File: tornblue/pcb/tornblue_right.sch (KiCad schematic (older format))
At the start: 80 parts, among them J1 BATT, J2 SWD, J3 BREAKOUT, J4 USB C - USB2.0, J5 BATT_PIN, Q1 AO3401A, Q2 AO3401A, SW1 SW_Push, SW10 SW_Push, SW11 SW_Push, SW12 SW_Push, SW13 SW_Push, SW14 SW_Push, SW15 SW_Push, SW16 SW_Push, SW17 SW_Push, SW18 SW_Push, SW19 EC11, SW2 SW_Push, SW20 SW_Push, SW21 SW_Push, SW22 EC11, SW23 RESET, SW24 SW_SPST, SW3 SW_Push, SW4 SW_Push, SW5 SW_Push, SW6 SW_Push, SW7 SW_Push, SW8 SW_Push, SW9 SW_Push, U1 XC6220, U2 TP4056, U3 nRF52840_holyiot_18010, U4 SRV05-4

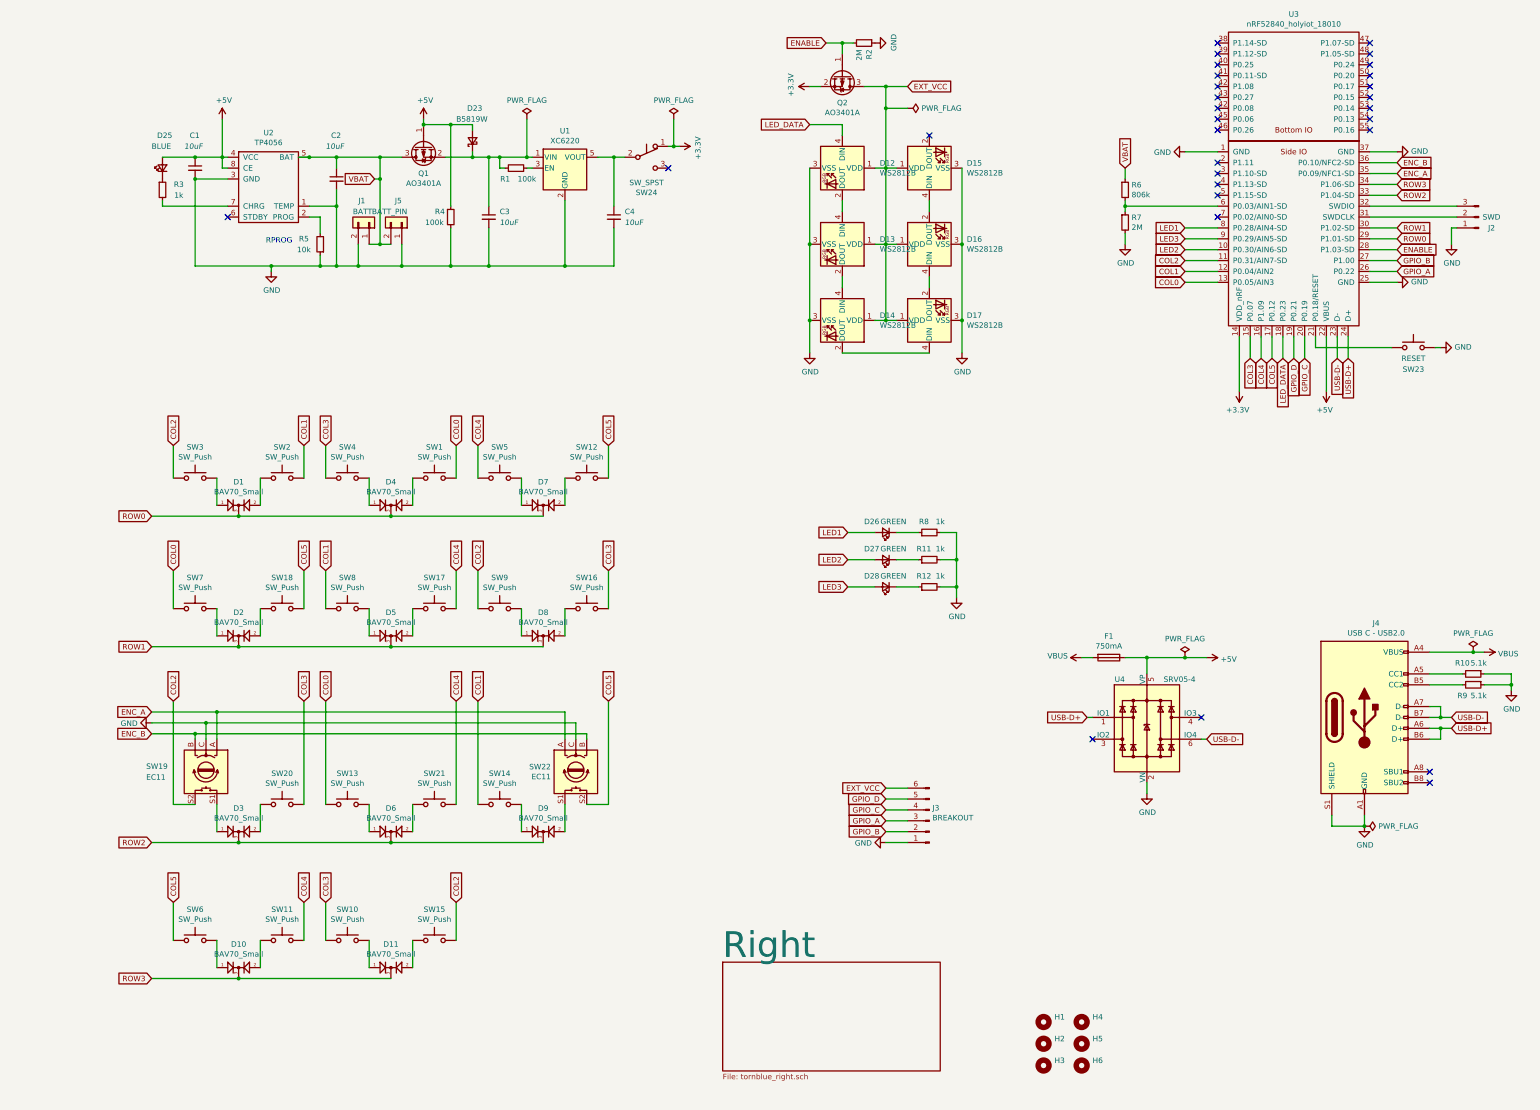
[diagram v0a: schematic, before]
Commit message: Add right schematic
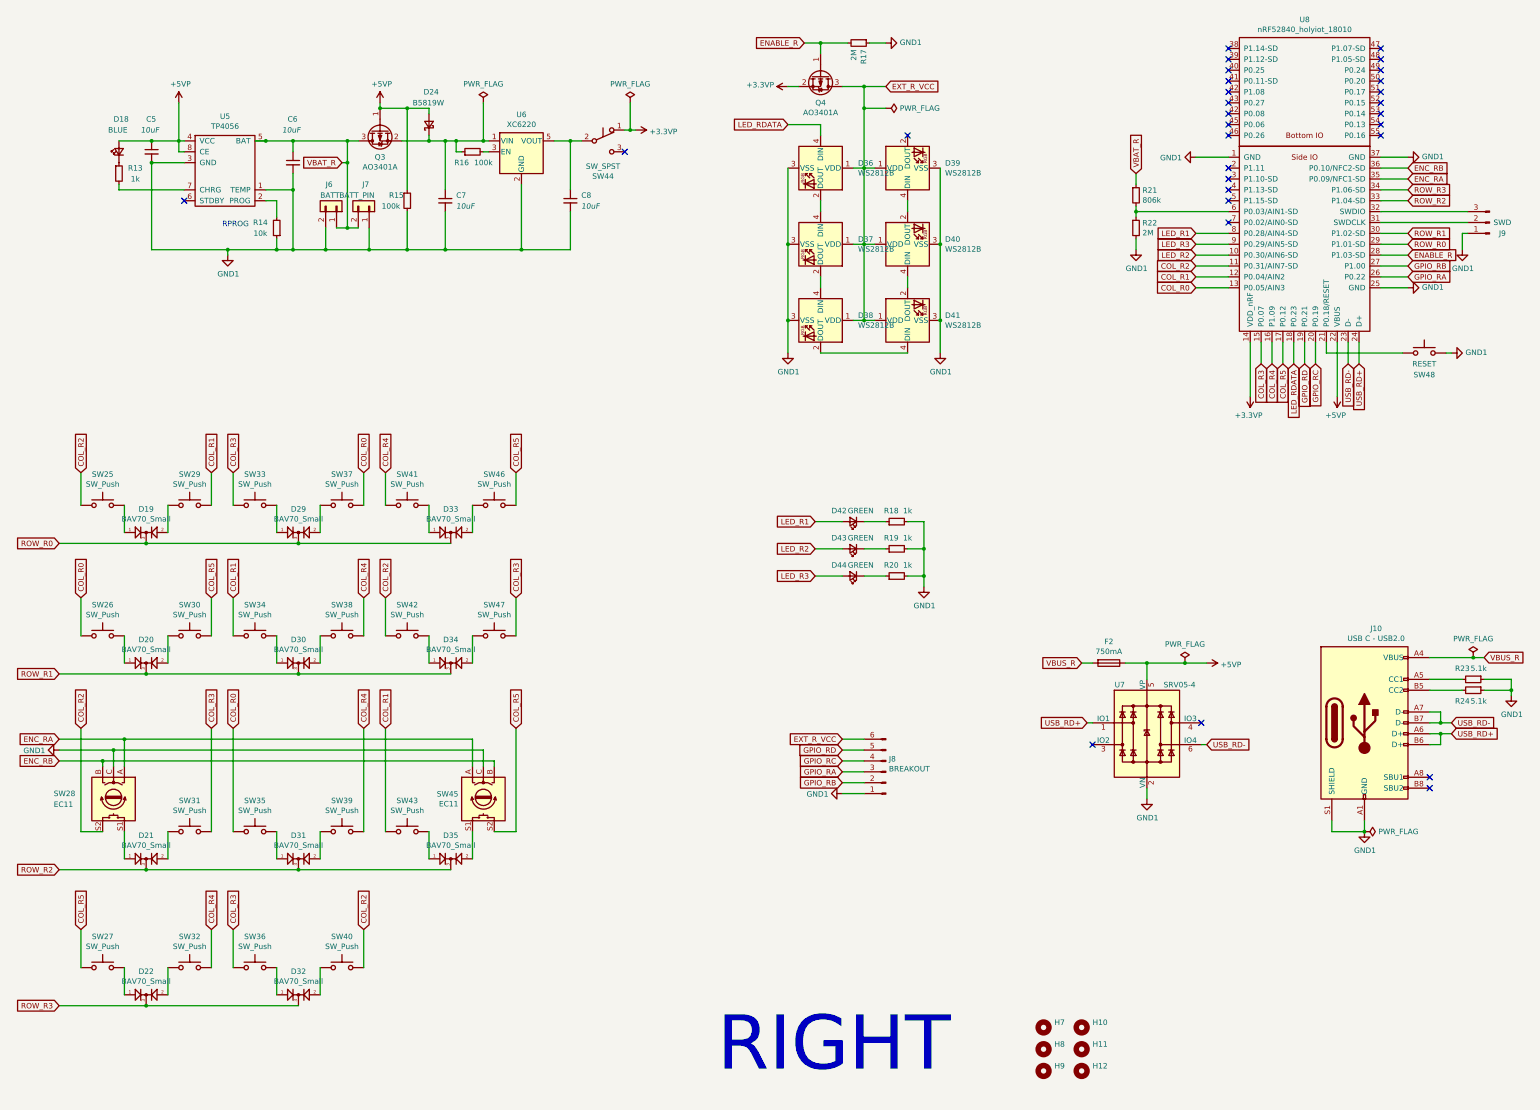
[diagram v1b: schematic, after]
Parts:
- removed C1, C2, C3, C4: 10uF, Diode_SMD:D_0805_2012Metric, symbol Device:C_Small
- removed D1, D10, D11, D2, D3, D4, D5, D6, D7, D8, D9: BAV70_Small, Package_TO_SOT_SMD:SOT-23, symbol kicad-keyboard-parts:BAV70_Small
- removed D12, D13, D14, D15, D16, D17: WS2812B, LED_SMD:LED_WS2812B_PLCC4_5.0x5.0mm_P3.2mm, symbol LED:WS2812B
- removed D23: B5819W, Diode_SMD:D_SOD-123, symbol Device:D_Schottky_Small
- removed D25: BLUE, LED_SMD:LED_0805_2012Metric, symbol Device:LED_Small
- removed D26, D27, D28: GREEN, LED_SMD:LED_0805_2012Metric, symbol Device:LED_Small
- removed F1: 750mA, Fuse:Fuse_1206_3216Metric, symbol Device:Fuse
- removed H1, H2, H3, H4: MountingHole, MountingHole:MountingHole_3.2mm_M3_DIN965_Pad, symbol Mechanical:MountingHole
- removed H5, H6: MountingHole, tornblue:MountingHole_3.2mm_M3_DIN965_Pad_Slot, symbol Mechanical:MountingHole
- removed J1: BATT, Connector_JST:JST_PH_S2B-PH-SM4-TB_1x02-1MP_P2.00mm_Horizontal, symbol Connector_Generic:Conn_01x02
- removed J2: SWD, tornblue:SOIC_clipProgSmall, symbol Connector:Conn_01x03_Male
- removed J3: BREAKOUT, Connector_PinHeader_1.27mm:PinHeader_1x06_P1.27mm_Vertical, symbol Connector:Conn_01x06_Male
- removed J4: USB C - USB2.0, Connector_USB:USB_C_Receptacle_XKB_U262-16XN-4BVC11, symbol Connector:USB_C_Receptacle_USB2.0
- removed J5: BATT_PIN, Connector_PinHeader_2.54mm:PinHeader_1x02_P2.54mm_Vertical, symbol Connector_Generic:Conn_01x02
- removed Q1, Q2: AO3401A, Package_TO_SOT_SMD:SOT-23, symbol Transistor_FET:AO3401A
- removed R1, R4: 100k, Resistor_SMD:R_0805_2012Metric, symbol Device:R_Small
- removed R10, R9: 5.1k, Resistor_SMD:R_0805_2012Metric, symbol Device:R_Small
- removed R11, R12, R3, R8: 1k, Resistor_SMD:R_0805_2012Metric, symbol Device:R_Small
- removed R2, R7: 2M, Resistor_SMD:R_0805_2012Metric, symbol Device:R_Small
- removed R5: 10k, Resistor_SMD:R_0805_2012Metric, symbol Device:R_Small
- removed R6: 806k, Resistor_SMD:R_0805_2012Metric, symbol Device:R_Small
- removed SW1, SW10, SW11, SW12, SW13, SW14, SW15, SW16, SW17, SW18, SW2, SW20, SW21, SW3, SW4, SW5, SW6, SW7, SW8, SW9: SW_Push, tornblue:MX_PG1350_optional, symbol Switch:SW_Push
- removed SW19, SW22: EC11, tornblue:MX_PG1350_EVQWGD001_LR_optional, symbol Device:Rotary_Encoder_Switch
- removed SW23: RESET, tornblue:SW_SPST_TS24CA, symbol Switch:SW_Push
- removed SW24: SW_SPST, Button_Switch_SMD:SW_SPDT_PCM12, symbol Switch:SW_Push_SPDT
- removed U1: XC6220, Package_TO_SOT_SMD:SOT-23-5, symbol Regulator_Linear:AP2112K-3.3
- removed U2: TP4056, Package_SO:SOIC-8-1EP_3.9x4.9mm_P1.27mm_EP2.29x3mm_ThermalVias, symbol kicad-keyboard-parts:TP4056
- removed U3: nRF52840_holyiot_18010, kicad-keyboard-parts:nRF52840_holyiot_18010, symbol tornblue-rescue:nRF52840_holyiot_18010-tornblue-tornblue-rescue
- removed U4: SRV05-4, Package_TO_SOT_SMD:SOT-23-6, symbol Power_Protection:SRV05-4
- added C5, C6, C7, C8: 10uF, Diode_SMD:D_0805_2012Metric, symbol Device:C_Small
- added D18: BLUE, LED_SMD:LED_0805_2012Metric, symbol Device:LED_Small
- added D19, D20, D21, D22, D29, D30, D31, D32, D33, D34, D35: BAV70_Small, Package_TO_SOT_SMD:SOT-23, symbol kicad-keyboard-parts:BAV70_Small
- added D24: B5819W, Diode_SMD:D_SOD-123, symbol Device:D_Schottky_Small
- added D36, D37, D38, D39, D40, D41: WS2812B, LED_SMD:LED_WS2812B_PLCC4_5.0x5.0mm_P3.2mm, symbol LED:WS2812B
- added D42, D43, D44: GREEN, LED_SMD:LED_0805_2012Metric, symbol Device:LED_Small
- added F2: 750mA, Fuse:Fuse_1206_3216Metric, symbol Device:Fuse
- added H10, H7, H8, H9: MountingHole, MountingHole:MountingHole_3.2mm_M3_DIN965_Pad, symbol Mechanical:MountingHole
- added H11, H12: MountingHole, tornblue:MountingHole_3.2mm_M3_DIN965_Pad_Slot, symbol Mechanical:MountingHole
- added J10: USB C - USB2.0, Connector_USB:USB_C_Receptacle_XKB_U262-16XN-4BVC11, symbol Connector:USB_C_Receptacle_USB2.0
- added J6: BATT, Connector_JST:JST_PH_S2B-PH-SM4-TB_1x02-1MP_P2.00mm_Horizontal, symbol Connector_Generic:Conn_01x02
- added J7: BATT_PIN, Connector_PinHeader_2.54mm:PinHeader_1x02_P2.54mm_Vertical, symbol Connector_Generic:Conn_01x02
- added J8: BREAKOUT, Connector_PinHeader_1.27mm:PinHeader_1x06_P1.27mm_Vertical, symbol Connector:Conn_01x06_Male
- added J9: SWD, tornblue:SOIC_clipProgSmall, symbol Connector:Conn_01x03_Male
- added Q3, Q4: AO3401A, Package_TO_SOT_SMD:SOT-23, symbol Transistor_FET:AO3401A
- added R13, R18, R19, R20: 1k, Resistor_SMD:R_0805_2012Metric, symbol Device:R_Small
- added R14: 10k, Resistor_SMD:R_0805_2012Metric, symbol Device:R_Small
- added R15, R16: 100k, Resistor_SMD:R_0805_2012Metric, symbol Device:R_Small
- added R17, R22: 2M, Resistor_SMD:R_0805_2012Metric, symbol Device:R_Small
- added R21: 806k, Resistor_SMD:R_0805_2012Metric, symbol Device:R_Small
- added R23, R24: 5.1k, Resistor_SMD:R_0805_2012Metric, symbol Device:R_Small
- added SW25, SW26, SW27, SW29, SW30, SW31, SW32, SW33, SW34, SW35, SW36, SW37, SW38, SW39, SW40, SW41, SW42, SW43, SW46, SW47: SW_Push, tornblue:MX_PG1350_optional, symbol Switch:SW_Push
- added SW28, SW45: EC11, tornblue:MX_PG1350_EVQWGD001_LR_optional, symbol Device:Rotary_Encoder_Switch
- added SW44: SW_SPST, Button_Switch_SMD:SW_SPDT_PCM12, symbol Switch:SW_Push_SPDT
- added SW48: RESET, tornblue:SW_SPST_TS24CA, symbol Switch:SW_Push
- added U5: TP4056, Package_SO:SOIC-8-1EP_3.9x4.9mm_P1.27mm_EP2.29x3mm_ThermalVias, symbol kicad-keyboard-parts:TP4056
- added U6: XC6220, Package_TO_SOT_SMD:SOT-23-5, symbol Regulator_Linear:AP2112K-3.3
- added U7: SRV05-4, Package_TO_SOT_SMD:SOT-23-6, symbol Power_Protection:SRV05-4
- added U8: nRF52840_holyiot_18010, kicad-keyboard-parts:nRF52840_holyiot_18010, symbol tornblue-rescue:nRF52840_holyiot_18010-tornblue-tornblue-rescue
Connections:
- new net: SW48.1, U8.21 (P0.18/RESET)
- new net: J9.2 (Pin_2), U8.31 (SWDCLK)
- new net: J9.3 (Pin_3), U8.32 (SWDIO)
- new net: R21.2, R22.1, U8.6 (P0.03/AIN1-SD)
- new net: D42.1 (K), R18.1
- new net: D43.1 (K), R19.1
- new net: D44.1 (K), R20.1
- new net: J10.B5 (CC2), R24.2
- new net: J10.A5 (CC1), R23.2
- new net: D18.1 (K), R13.1
- new net: R13.2, U5.7 (CHRG)
- new net: R14.2, U5.2 (PROG)
- new net: C7.1, D24.1 (K), Q3.2 (S), R16.1, U6.1 (VIN)
- new net: R16.2, U6.3 (EN)
- new net: C8.1, SW44.2 (B), U6.5 (VOUT)
- new net: D36.2 (DOUT), D37.4 (DIN)
- new net: D37.2 (DOUT), D38.4 (DIN)
- new net: D38.2 (DOUT), D41.4 (DIN)
- new net: D40.4 (DIN), D41.2 (DOUT)
- new net: D39.4 (DIN), D40.2 (DOUT)
- new net: D22.1 (A1), SW27.2
- new net: D22.2 (A2), SW32.2
- new net: D30.2 (A2), SW38.2
- new net: D20.2 (A2), SW30.2
- new net: D35.2 (A2), SW45.S1
- new net: D30.1 (A1), SW34.2
- new net: D31.1 (A1), SW35.2
- new net: D31.2 (A2), SW39.2
- new net: D35.1 (A1), SW43.2
- new net: D21.1 (A1), SW28.S1
- new net: D34.1 (A1), SW42.2
- new net: D20.1 (A1), SW26.2
- new net: D21.2 (A2), SW31.2
- new net: D19.1 (A1), SW25.2
- new net: D19.2 (A2), SW29.2
- new net: D33.1 (A1), SW41.2
- new net: D33.2 (A2), SW46.2
- new net: D29.1 (A1), SW33.2
- new net: D29.2 (A2), SW37.2
- new net: D32.2 (A2), SW40.2
- new net: D34.2 (A2), SW47.2
- new net: D32.1 (A1), SW36.2
- new net +3.3VP: Q4.2 (S), SW44.1 (A), U8.14 (VDD_nRF)
- new net +5VP: C5.1, D18.2 (A), D24.2 (A), F2.1, Q3.1 (G), R15.1, U5.4 (VCC), U5.8 (CE), U7.5 (VP), U8.22 (VBUS)
- new net COL_R0: SW26.1, SW35.1, SW37.1, U8.13 (P0.05/AIN3)
- new net COL_R1: SW29.1, SW34.1, SW43.1, U8.12 (P0.04/AIN2)
- new net COL_R2: SW25.1, SW28.S2, SW40.1, SW42.1, U8.11 (P0.31/AIN7-SD)
- new net COL_R3: SW31.1, SW33.1, SW36.1, SW47.1, U8.15 (P0.07)
- new net COL_R4: SW32.1, SW38.1, SW39.1, SW41.1, U8.16 (P1.09)
- new net COL_R5: SW27.1, SW30.1, SW45.S2, SW46.1, U8.17 (P0.12)
- new net ENABLE_R: Q4.1 (G), R17.2, U8.28 (P1.03-SD)
- new net ENC_RA: SW28.A, SW45.A, U8.35 (P0.09/NFC1-SD)
- new net ENC_RB: SW28.B, SW45.B, U8.36 (P0.10/NFC2-SD)
- new net EXT_R_VCC: D36.1 (VDD), D37.1 (VDD), D38.1 (VDD), D39.1 (VDD), D40.1 (VDD), D41.1 (VDD), J8.6 (Pin_6), Q4.3 (D)
- new net GND1: C5.2, C6.2, C7.2, C8.2, D36.3 (VSS), D37.3 (VSS), D38.3 (VSS), D39.3 (VSS), D40.3 (VSS), D41.3 (VSS), J10.A1 (GND), J10.A12 (GND), J10.B1 (GND), J10.B12 (GND), J10.S1 (SHIELD), J6.2 (Pin_2), J7.1 (Pin_1), J8.1 (Pin_1), J9.1 (Pin_1), R14.1, R15.2, R17.1, R18.2, R19.2, R20.2, R22.2, R23.1, R24.1, SW28.C, SW45.C, SW48.2, U5.1 (TEMP), U5.3 (GND), U6.2 (GND), U7.2 (VN), U8.1 (GND), U8.25 (GND), U8.37 (GND)
- new net GPIO_RA: J8.3 (Pin_3), U8.26 (P0.22)
- new net GPIO_RB: J8.2 (Pin_2), U8.27 (P1.00)
- new net GPIO_RC: J8.4 (Pin_4), U8.20 (P0.19)
- new net GPIO_RD: J8.5 (Pin_5), U8.19 (P0.21)
- new net LED_R1: D42.2 (A), U8.8 (P0.28/AIN4-SD)
- new net LED_R2: D43.2 (A), U8.10 (P0.30/AIN6-SD)
- new net LED_R3: D44.2 (A), U8.9 (P0.29/AIN5-SD)
- new net LED_RDATA: D36.4 (DIN), U8.18 (P0.23)
- new net ROW_R0: D19.3 (K), D29.3 (K), D33.3 (K), U8.29 (P1.01-SD)
- new net ROW_R1: D20.3 (K), D30.3 (K), D34.3 (K), U8.30 (P1.02-SD)
- new net ROW_R2: D21.3 (K), D31.3 (K), D35.3 (K), U8.33 (P1.04-SD)
- new net ROW_R3: D22.3 (K), D32.3 (K), U8.34 (P1.06-SD)
- new net USB_RD+: J10.A6 (D+), J10.B6 (D+), U7.1 (IO1), U8.24 (D+)
- new net USB_RD-: J10.A7 (D-), J10.B7 (D-), U7.6 (IO4), U8.23 (D-)
- new net VBAT_R: C6.1, J6.1 (Pin_1), J7.2 (Pin_2), Q3.3 (D), R21.1, U5.5 (BAT)
- new net VBUS_R: F2.2, J10.A4 (VBUS), J10.A9 (VBUS), J10.B4 (VBUS), J10.B9 (VBUS)
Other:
- note added: "RIGHT"
